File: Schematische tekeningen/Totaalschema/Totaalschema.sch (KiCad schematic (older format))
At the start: 22 parts, among them IC1 MSP430FR2476TPTR, J1 Programmeer header, J10 ALL GPIO_1, J11 ALL GPIO_2, J12 3.3V pwr, J2 Labconnector +, J3 Labconnector -, J4 Display, J5 Motor-, J6 Motor+, J7 Breakoutbord, SW1 SW_Push, U1 74HC14, U14 Snelheidssensor

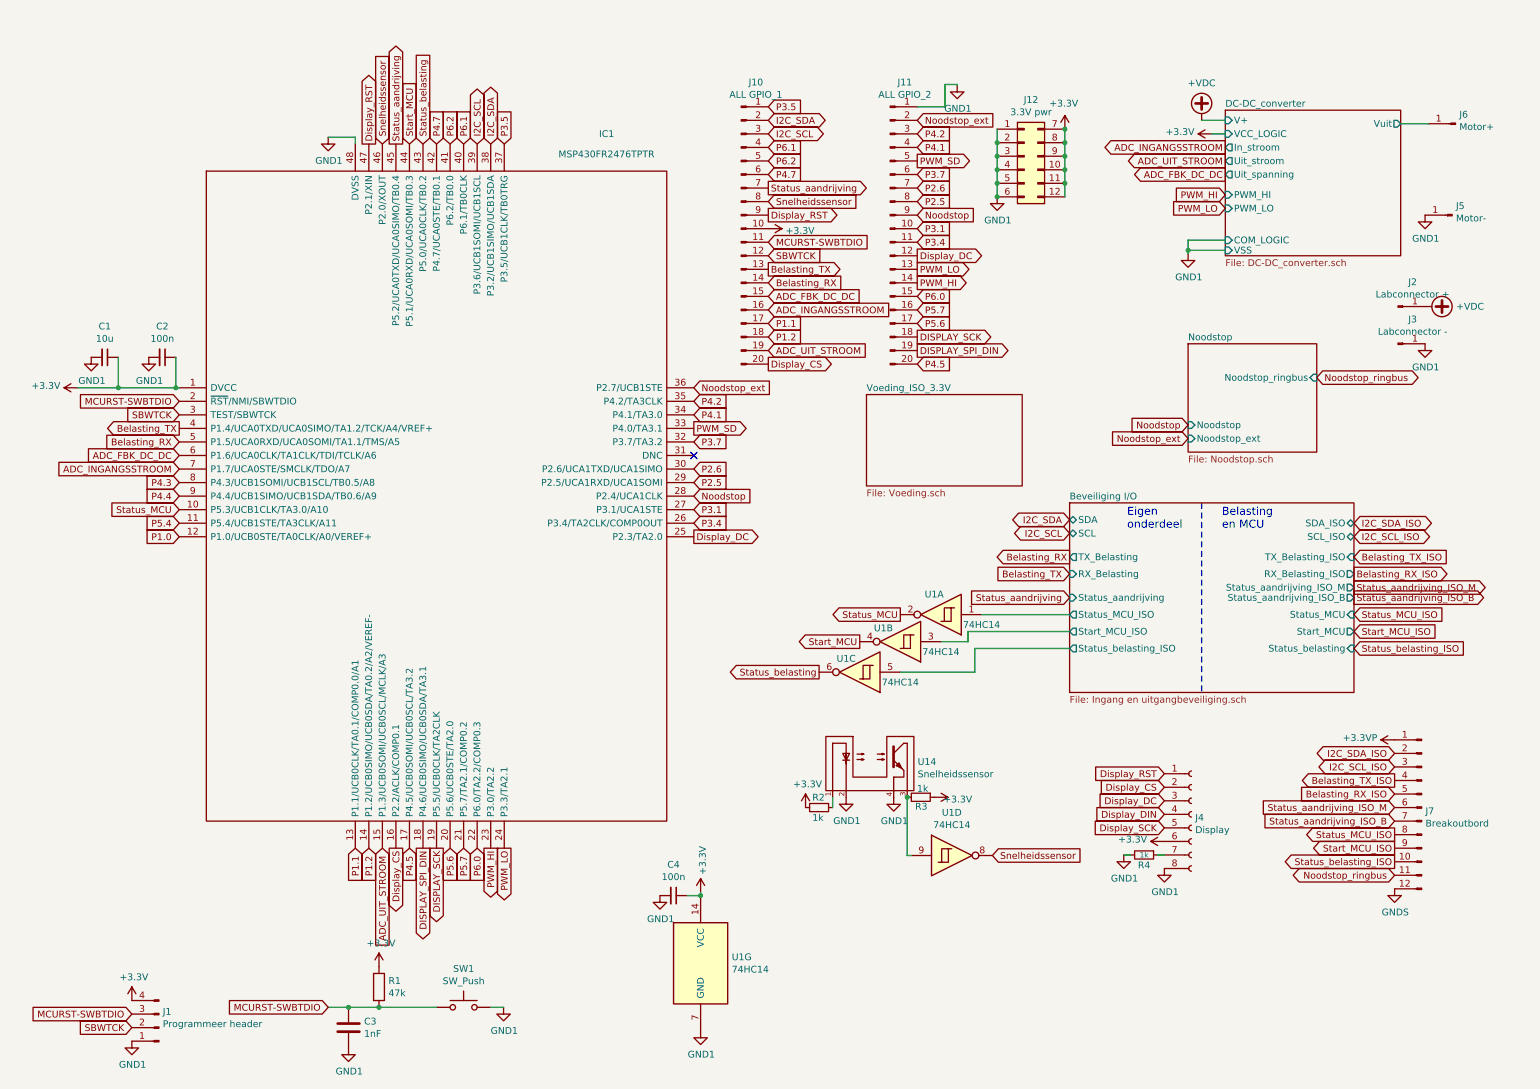
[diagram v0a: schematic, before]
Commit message: Totaalschema in orde maken
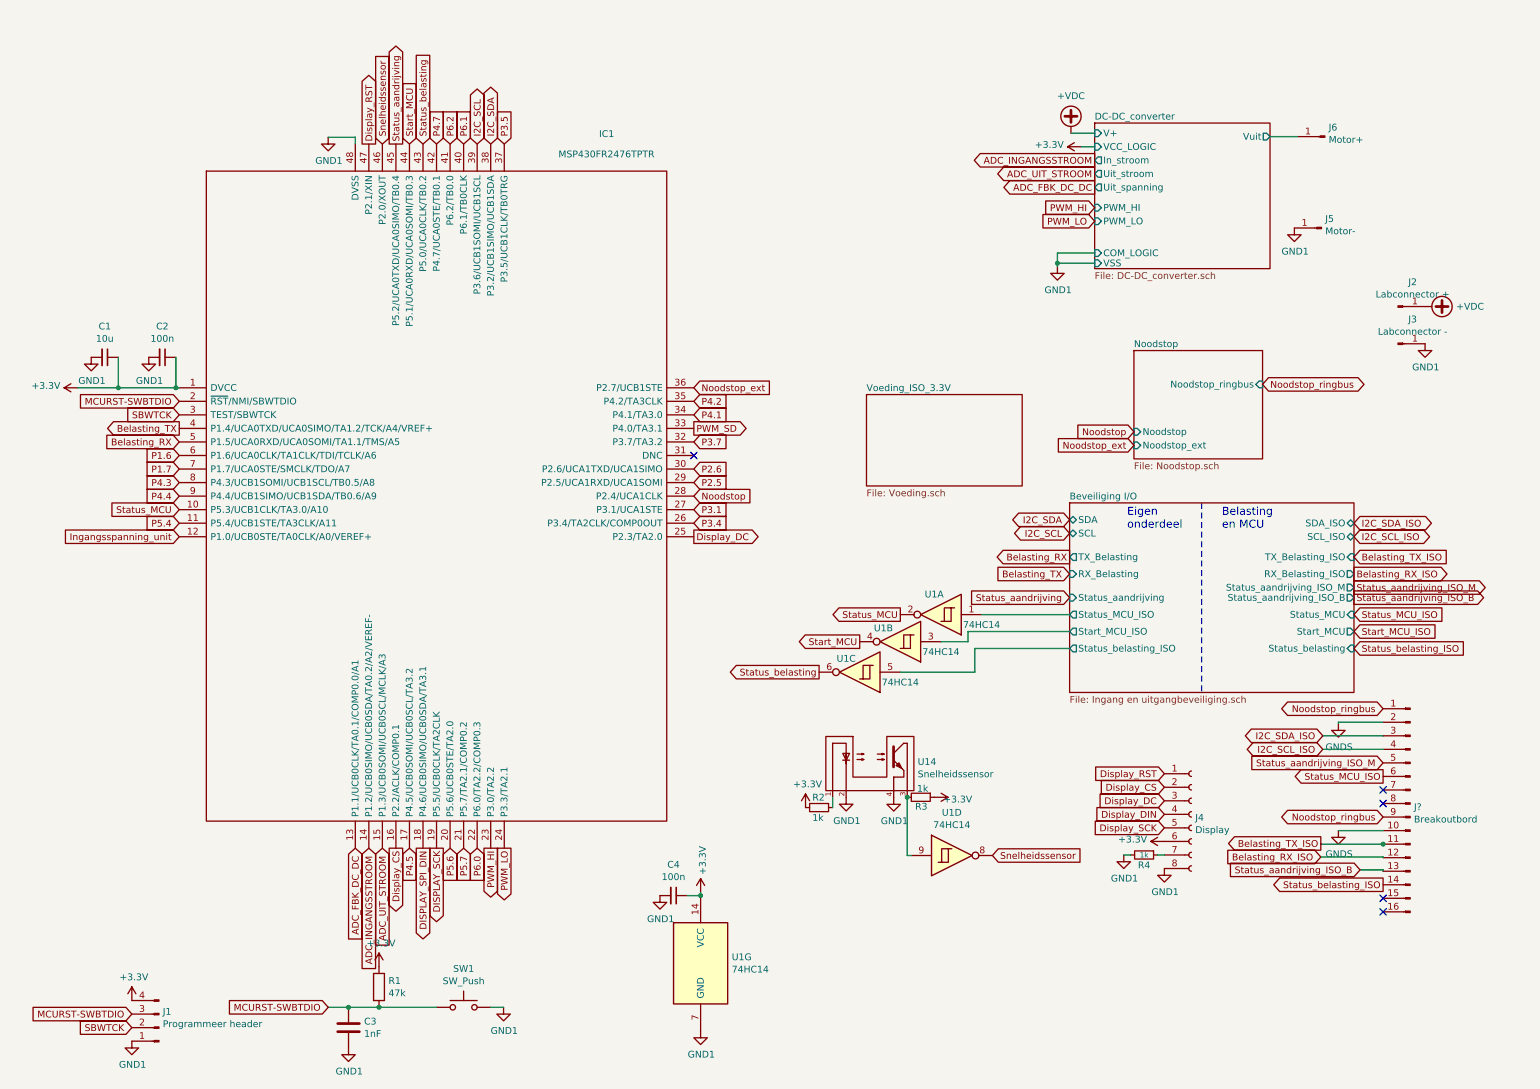
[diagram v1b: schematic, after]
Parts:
- removed J10: ALL GPIO_1, Connector_PinHeader_2.54mm:PinHeader_2x10_P2.54mm_Vertical_SMD, symbol Connector:Conn_01x20_Male
- removed J11: ALL GPIO_2, Connector_PinHeader_2.54mm:PinHeader_2x10_P2.54mm_Vertical_SMD, symbol Connector:Conn_01x20_Male
- removed J12: 3.3V pwr, Connector_PinHeader_2.54mm:PinHeader_2x06_P2.54mm_Vertical_SMD, symbol Connector_Generic:Conn_02x06_Top_Bottom
- removed J7: Breakoutbord, Connector_PinHeader_2.54mm:PinHeader_1x12_P2.54mm_Vertical, symbol Connector:Conn_01x12_Male
- added J?: Breakoutbord, symbol Connector:Conn_01x16_Male
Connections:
- net P1.1 is gone; now on net ADC_FBK_DC_DC: IC1.13 (P1.1/UCB0CLK/TA0.1/COMP0.0/A1)
- net P1.2 is gone; now on net ADC_INGANGSSTROOM: IC1.14 (P1.2/UCB0SIMO/UCB0SDA/TA0.2/A2/VEREF-)
- net ADC_FBK_DC_DC: no longer IC1.6 (P1.6/UCA0CLK/TA1CLK/TDI/TCLK/A6)
- net ADC_INGANGSSTROOM: no longer IC1.7 (P1.7/UCA0STE/SMCLK/TDO/A7)
- net Belasting_RX_ISO: now also J?.12 (Pin_12)
- net Belasting_TX_ISO: now also J?.11 (Pin_11)
- net GNDS: now also J?.10 (Pin_10), J?.2 (Pin_2)
- net I2C_SCL_ISO: now also J?.4 (Pin_4)
- net I2C_SDA_ISO: now also J?.3 (Pin_3)
- net Noodstop_ringbus: now also J?.1 (Pin_1), J?.9 (Pin_9)
- net Status_MCU_ISO: now also J?.6 (Pin_6)
- net Status_aandrijving_ISO_B: now also J?.13 (Pin_13)
- net Status_aandrijving_ISO_M: now also J?.5 (Pin_5)
- net Status_belasting_ISO: now also J?.14 (Pin_14)
- net P1.0 renamed Ingangsspanning_unit
- new net P1.6: IC1.6 (P1.6/UCA0CLK/TA1CLK/TDI/TCLK/A6)
- new net P1.7: IC1.7 (P1.7/UCA0STE/SMCLK/TDO/A7)
- no-connect marks 1 -> 5
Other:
- moved on the sheet: J5, J6
